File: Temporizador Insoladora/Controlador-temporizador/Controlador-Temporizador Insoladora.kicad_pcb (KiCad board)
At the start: 2 copper layers, 170.2 x 96.5 mm, 72 parts, among them P1 ICSP, P2 CONN_01X03, P3 CARGA, P4 TRANSF, P5 VAC, P7 CONN_02X08, Q1 BC548, Q2 BC548, Q3 BC548, Q4 BC548, Q5 BC548, Q6 BC548, SW1 Reset, SW2 SUBIR, SW3 BAJAR, SW4 GPI1, SW5 INICIAR/PARAR, U1 7805, U2 PIC16f871, U3 MOC3031M, U4 TRIAC, Y1 Crystal_Small

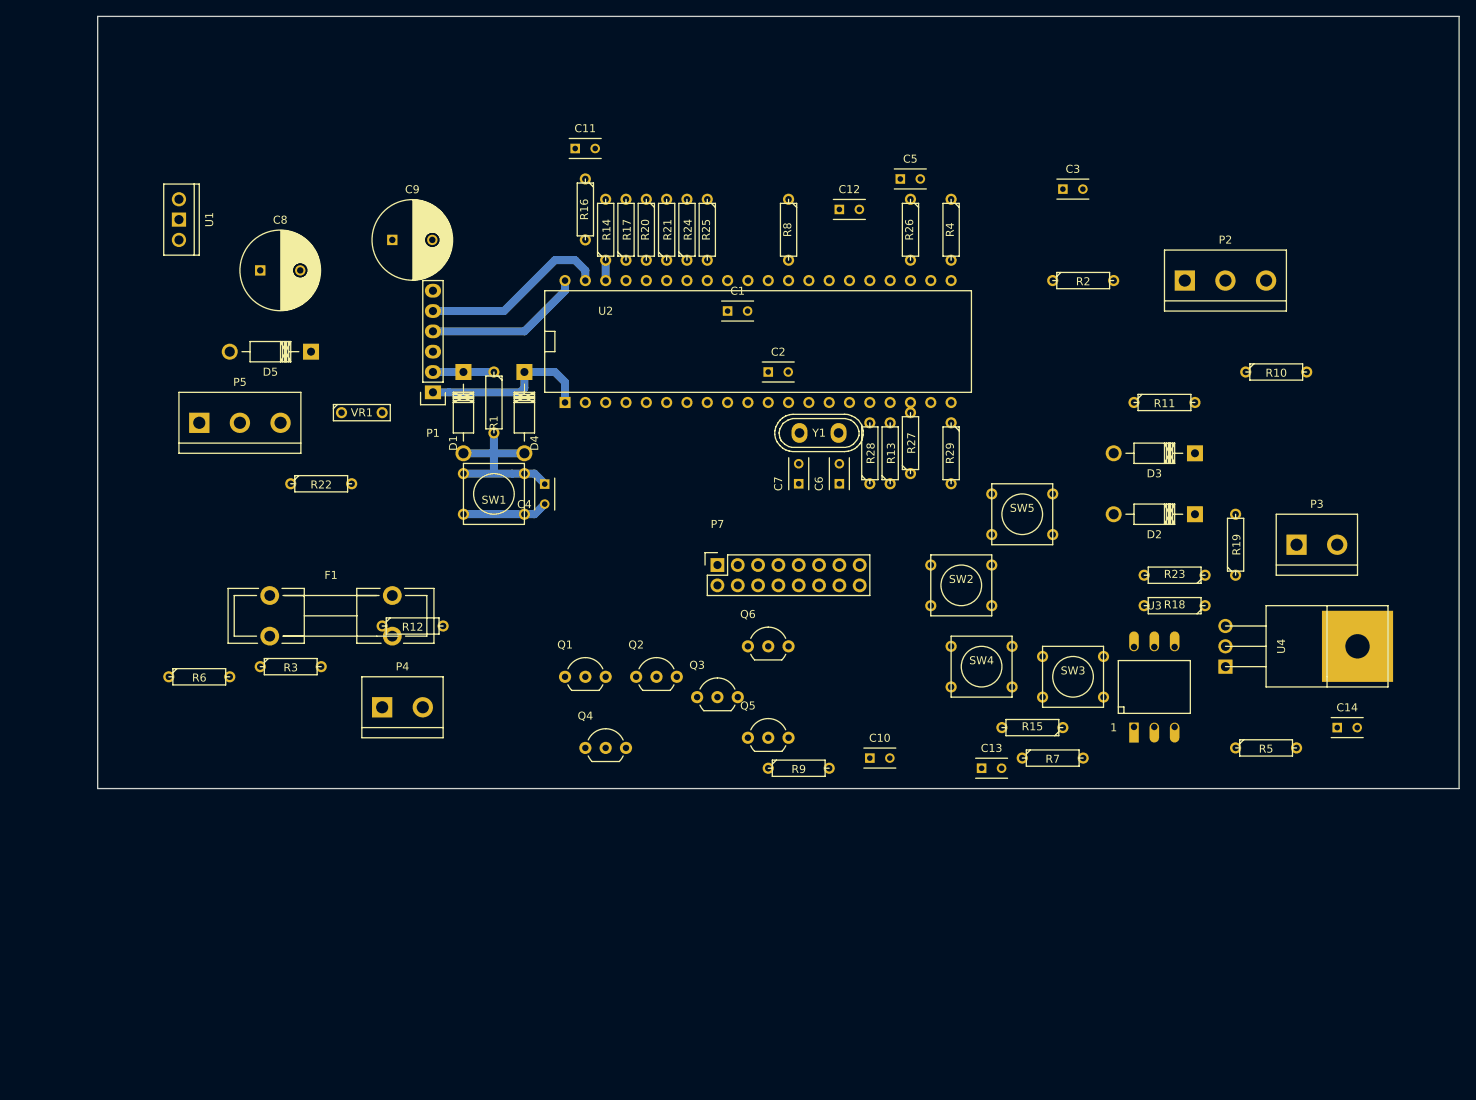
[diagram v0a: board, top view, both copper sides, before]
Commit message: Sigo ruteando pcb controlador insoladora
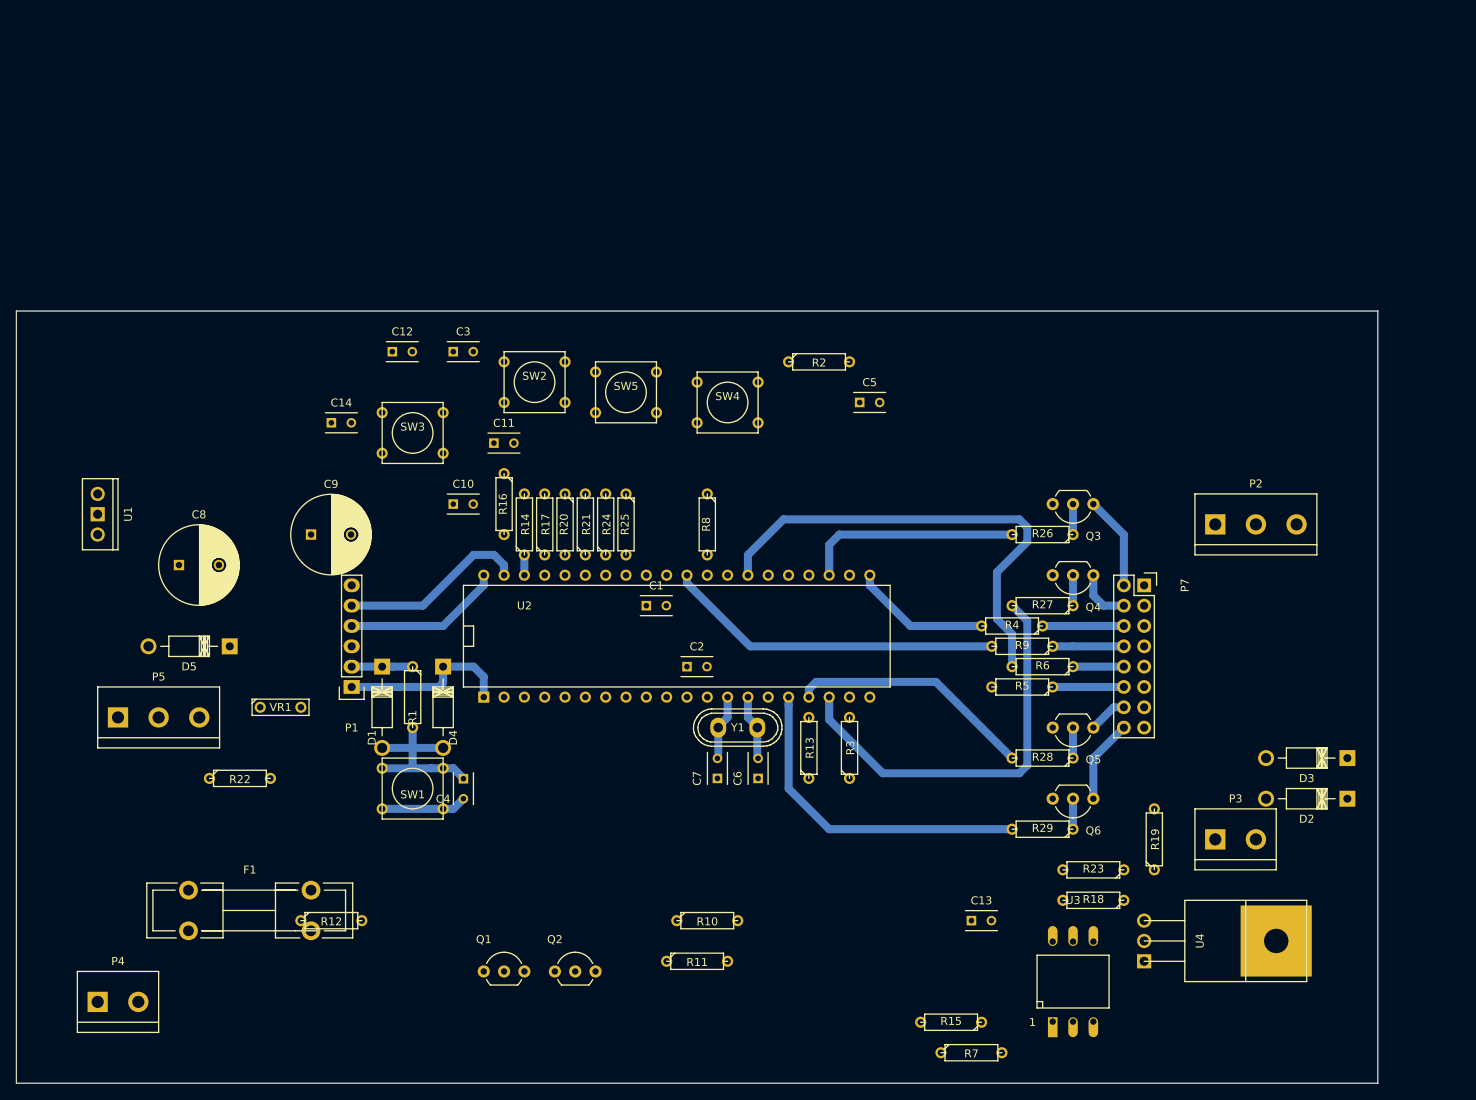
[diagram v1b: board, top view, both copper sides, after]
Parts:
- moved C14 131.4 mm to (80.0, 73.7)
- moved R6 105.4 mm to (168.9, 104.1), turned to 180 degrees
- moved R10 98.8 mm to (127.0, 135.9)
- moved R11 91.1 mm to (125.7, 141.0)
- moved SW3 88.0 mm to (90.2, 74.9)
- moved C3 78.9 mm to (95.2, 64.8)
- moved R3 70.6 mm to (144.8, 114.3), turned to 90 degrees
- moved Q4 67.1 mm to (175.3, 92.7), turned to 180 degrees
- moved C10 61.0 mm to (95.2, 83.8)
- moved SW2 59.1 mm to (105.4, 68.6)
- moved C12 58.6 mm to (87.6, 64.8)
- moved Q3 55.1 mm to (175.3, 83.8), turned to 180 degrees
- moved P7 53.4 mm to (181.6, 94.0), turned to 270 degrees
- moved SW5 51.8 mm to (116.8, 69.8)
- moved P4 51.2 mm to (53.3, 146.1)
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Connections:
- P1 pad 6: Net-(P1-Pad6) -> (no net)
- P5 pad 2: Earth -> (no net)
- P7 pad 11: Net-(P7-Pad11) -> (no net)
- P7 pad 5: Net-(P7-Pad5) -> (no net)
- P7 pad 7: Net-(P7-Pad7) -> (no net)
- P7 pad 9: Net-(P7-Pad9) -> (no net)
- Q1 pad 1: MINDKC -> Net-(Q1-Pad1)
- Q3 pad 1: Net-(Q3-Pad1) -> MINDKC
- R13 pad 1: Net-(Q3-Pad2) -> Net-(Q1-Pad2)
- R15 pad 2: Net-(Q3-Pad1) -> Net-(Q1-Pad1)
- R26 pad 1: Net-(Q1-Pad2) -> Net-(Q3-Pad2)
- U2 pad 10: Net-(U2-Pad10) -> (no net)
- U2 pad 2: Net-(U2-Pad2) -> (no net)
- U2 pad 24: Net-(U2-Pad24) -> (no net)
- U2 pad 25: Net-(U2-Pad25) -> (no net)
- U2 pad 26: Net-(U2-Pad26) -> (no net)
- U2 pad 3: Net-(U2-Pad3) -> (no net)
- U2 pad 34: Net-(U2-Pad34) -> (no net)
- U2 pad 4: Net-(U2-Pad4) -> (no net)
- U2 pad 5: Net-(U2-Pad5) -> (no net)
- U2 pad 6: Net-(U2-Pad6) -> (no net)
- U2 pad 7: Net-(U2-Pad7) -> (no net)
- U2 pad 8: Net-(U2-Pad8) -> (no net)
- U2 pad 9: Net-(U2-Pad9) -> (no net)
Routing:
- net /RD4: track 0.00 -> 59.5 mm
- net MINU: track 0.00 -> 51.5 mm
- net /RD7: track 0.00 -> 42.4 mm
- net SEGU: track 0.00 -> 41.5 mm
- net SEGD: track 0.00 -> 30.7 mm
- net MIND: track 0.00 -> 27.2 mm
- net /RD2: track 0.00 -> 17.3 mm
- net MINDKC: track 0.00 -> 11.7 mm
- net SEGUKC: track 0.00 -> 10.5 mm
- net /C: track 0.00 -> 10.2 mm
- net /DP: track 0.00 -> 8.89 mm
- net /D: track 0.00 -> 8.89 mm
- net Net-(C7-Pad2): track 0.00 -> 8.19 mm
- net Net-(C6-Pad2): track 0.00 -> 8.19 mm
- net MINUKC: track 0.00 -> 6.88 mm
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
